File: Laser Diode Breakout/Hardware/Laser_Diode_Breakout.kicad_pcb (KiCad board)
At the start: 2 copper layers, 29.2 x 35.6 mm, 10 parts, among them Q1 BSS138, Q2 BSS138

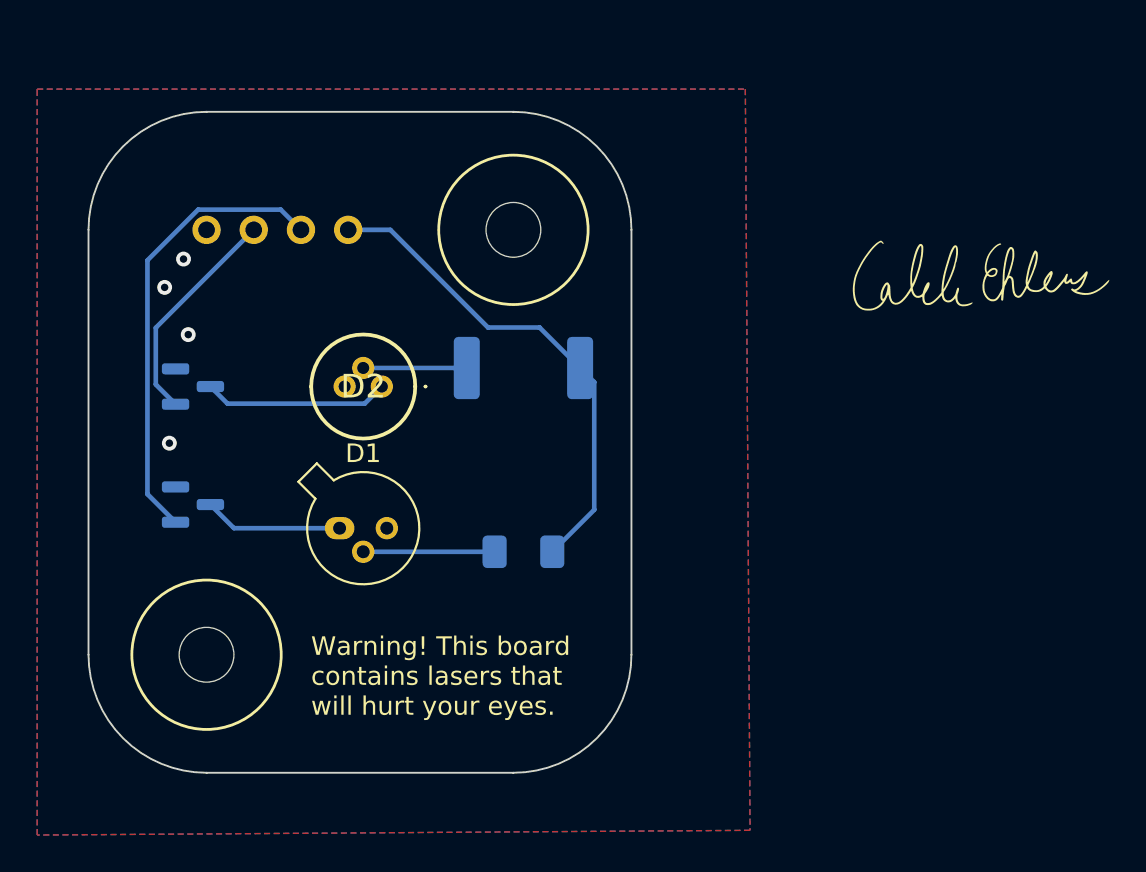
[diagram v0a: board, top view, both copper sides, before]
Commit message: finish diode breakout changes
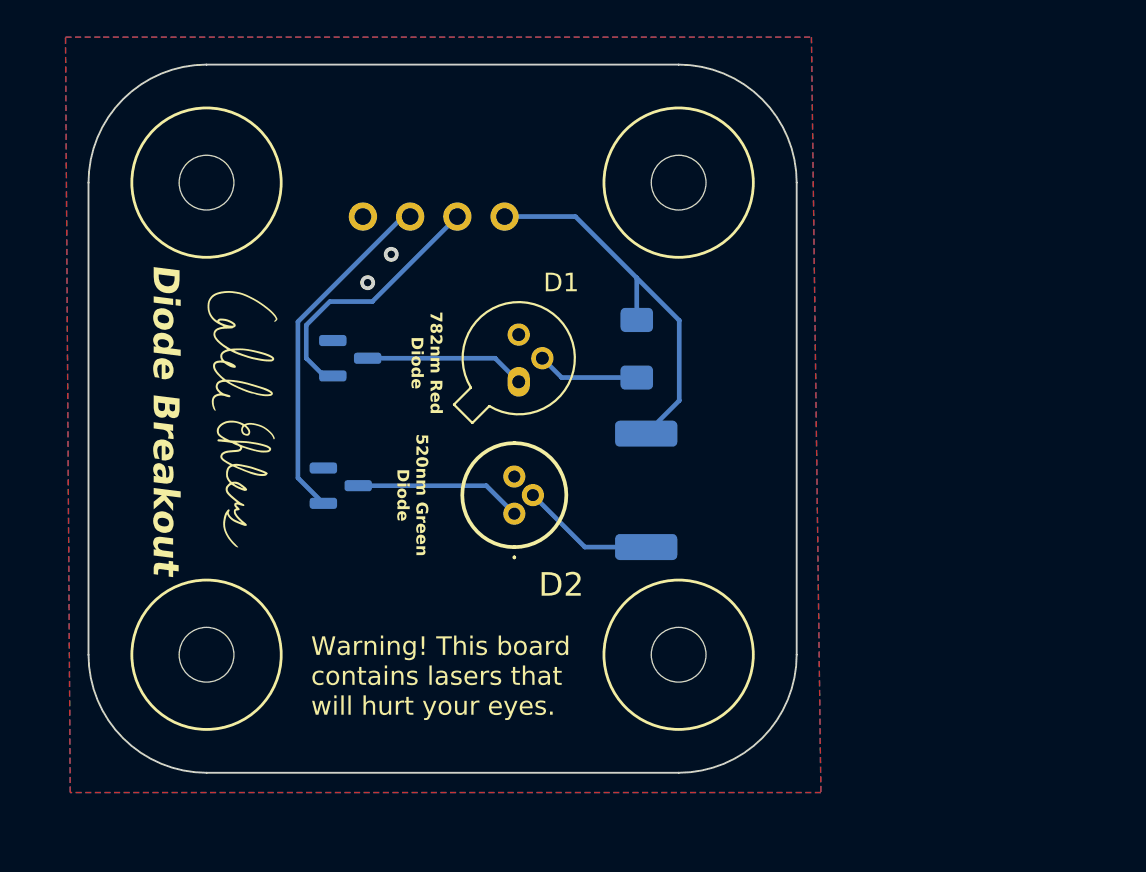
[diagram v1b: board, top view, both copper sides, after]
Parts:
- added V3: Via, MRDT_Drill_Holes:4_40_Hole, F.Cu at (36.3, 33.5)
- added V4: Via, MRDT_Drill_Holes:4_40_Hole, F.Cu at (61.7, 58.9)
- D1: value 785nm Laser Diode -> 782nm Laser Diode
- moved G*** 40.4 mm to (38.4, 46.2), turned to -90 degrees
- moved R2 12.5 mm to (59.4, 42.4), turned to -90 degrees
- moved D1 12.4 mm to (53.1, 44.2), turned to 90 degrees
- moved Q2 11.6 mm to (44.0, 42.9)
- moved D2 9.88 mm to (52.8, 51.3), turned to 90 degrees
- moved Q1 9.58 mm to (43.5, 49.8)
- moved R1 9.32 mm to (59.9, 50.0), turned to -90 degrees
- moved V1 9.25 mm to (61.7, 33.5)
- moved Conn1 8.44 mm to (52.3, 35.3)
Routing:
- net Red_LED: track 24.6 -> 14.1 mm
- net Green_LED: track 12.0 -> 18.7 mm
- net +12V: track 26.7 -> 20.8 mm
- net Net-(D2-A): track 5.57 -> 7.25 mm
- net Net-(D1-A): track 7.07 -> 5.51 mm
- net Net-(D1-K): track 7.48 -> 8.65 mm
- net Net-(D2-K): track 9.99 -> 9.02 mm
- net GND: vias 4 -> 2
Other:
- board size 29.2 x 35.6 mm -> 38.1 x 38.1 mm
- board text added: "520nm Green Diode"
- board text added: "782nm Red Diode"
- board text added: "Diode Breakout"
